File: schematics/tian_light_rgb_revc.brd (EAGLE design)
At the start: 7 parts

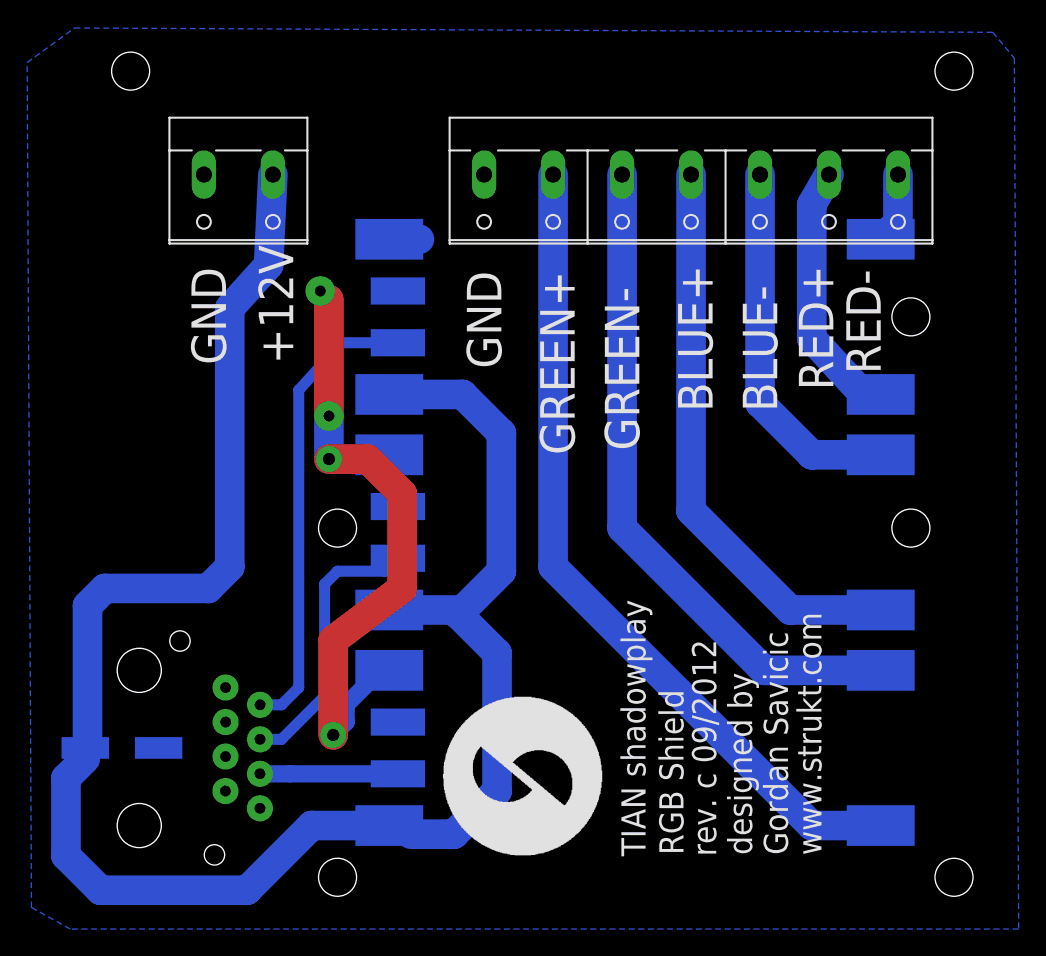
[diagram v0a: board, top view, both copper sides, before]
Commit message: -a
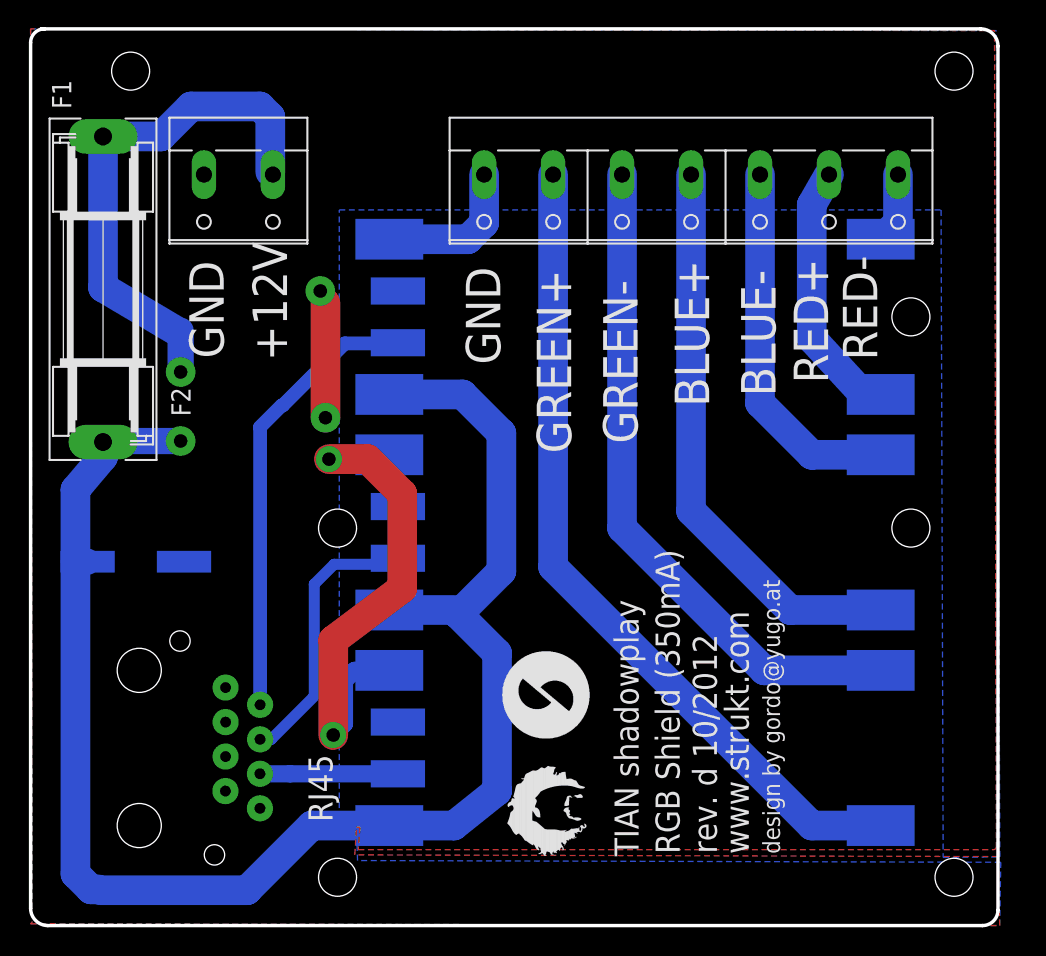
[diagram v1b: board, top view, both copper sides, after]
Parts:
- removed C1: (no value), rcl:153CLV-0605
- added C2: 220uF, rcl:PANASONIC_F
- added F1: (no value), fuse:SH22,5
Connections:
- new net N$1: F1.1, X1.1
- net 12V: now also C2.+, F1.2; no longer C1.+, X1.1
- net GND: now also C2.-; no longer C1.-
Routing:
- net N$1: track 0.00 -> 34.9 mm
- net 12V: track 142.7 -> 113.9 mm
- net GND: track 53.1 -> 59.8 mm
- net N$2: track 0.00 -> 5.59 mm, vias 0 -> 1
- net N$3: track 0.00 -> 3.05 mm, vias 0 -> 1
- net PWM_RED: track 34.1 -> 33.1 mm
- added copper zone on layer 1, net GND
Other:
- board outline added: 71.2 x 66 mm
- board text added: "F1"
- board text added: "F2"
- board text added: "RGB Shield (350mA)"
- board text added: "RJ45"
- board text added: "design by gordo@yugo.at"
- board text added: "rev. d 10/2012"
- board text removed: "Gordan Savicic"
- board text removed: "RGB Shield"
- board text removed: "designed by"
- board text removed: "rev. c 09/2012"
